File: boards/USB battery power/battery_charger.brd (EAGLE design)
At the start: 160 x 100 mm, 6 parts, among them IC1 MAX1555, U1 MAX8934EETI+, U2 LTC3127EMSEPBF

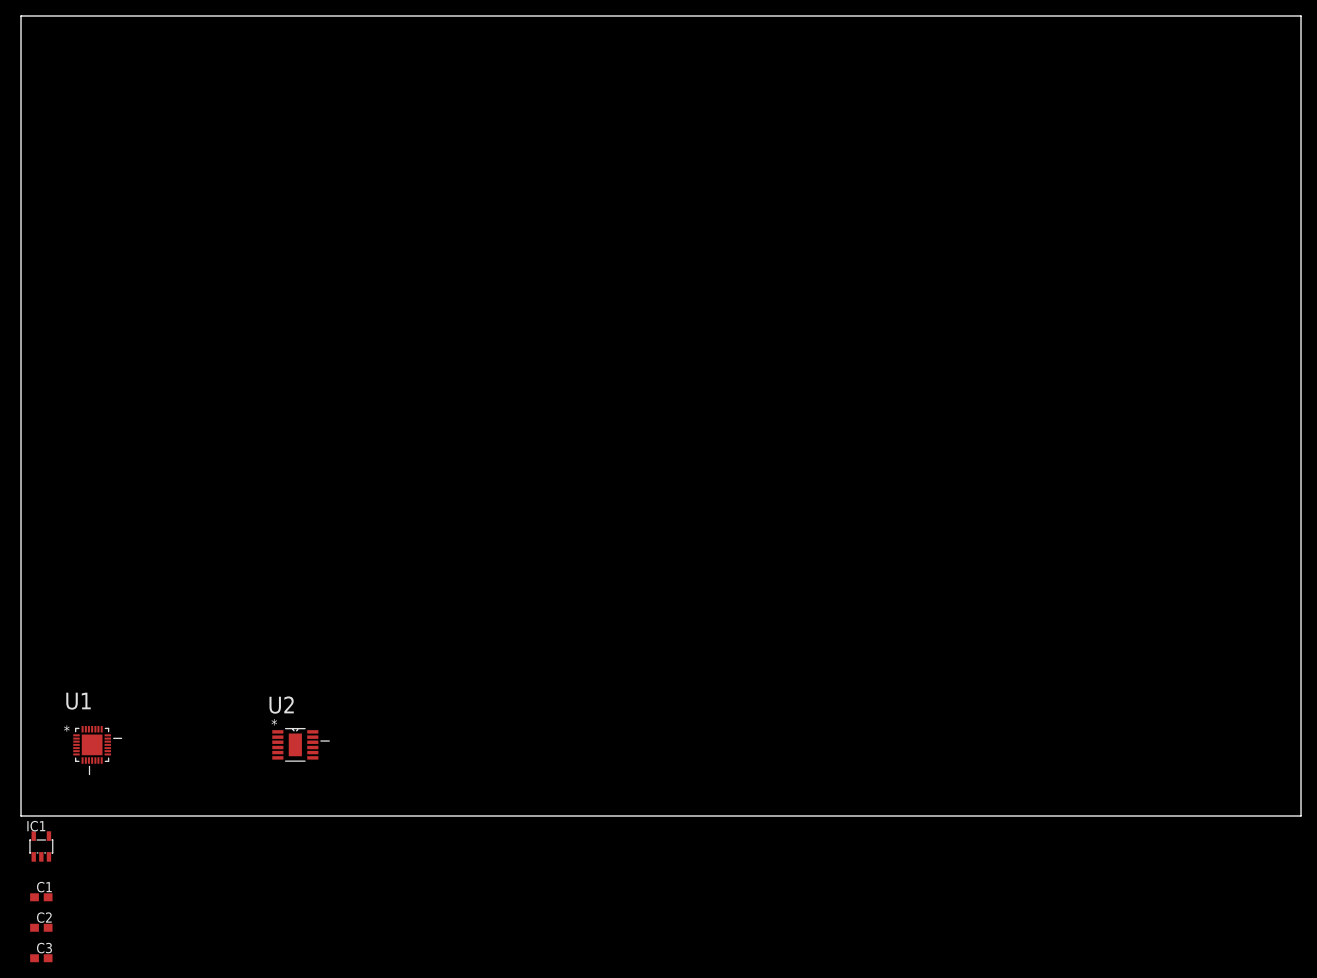
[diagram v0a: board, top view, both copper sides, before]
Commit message: Battery Charger test board
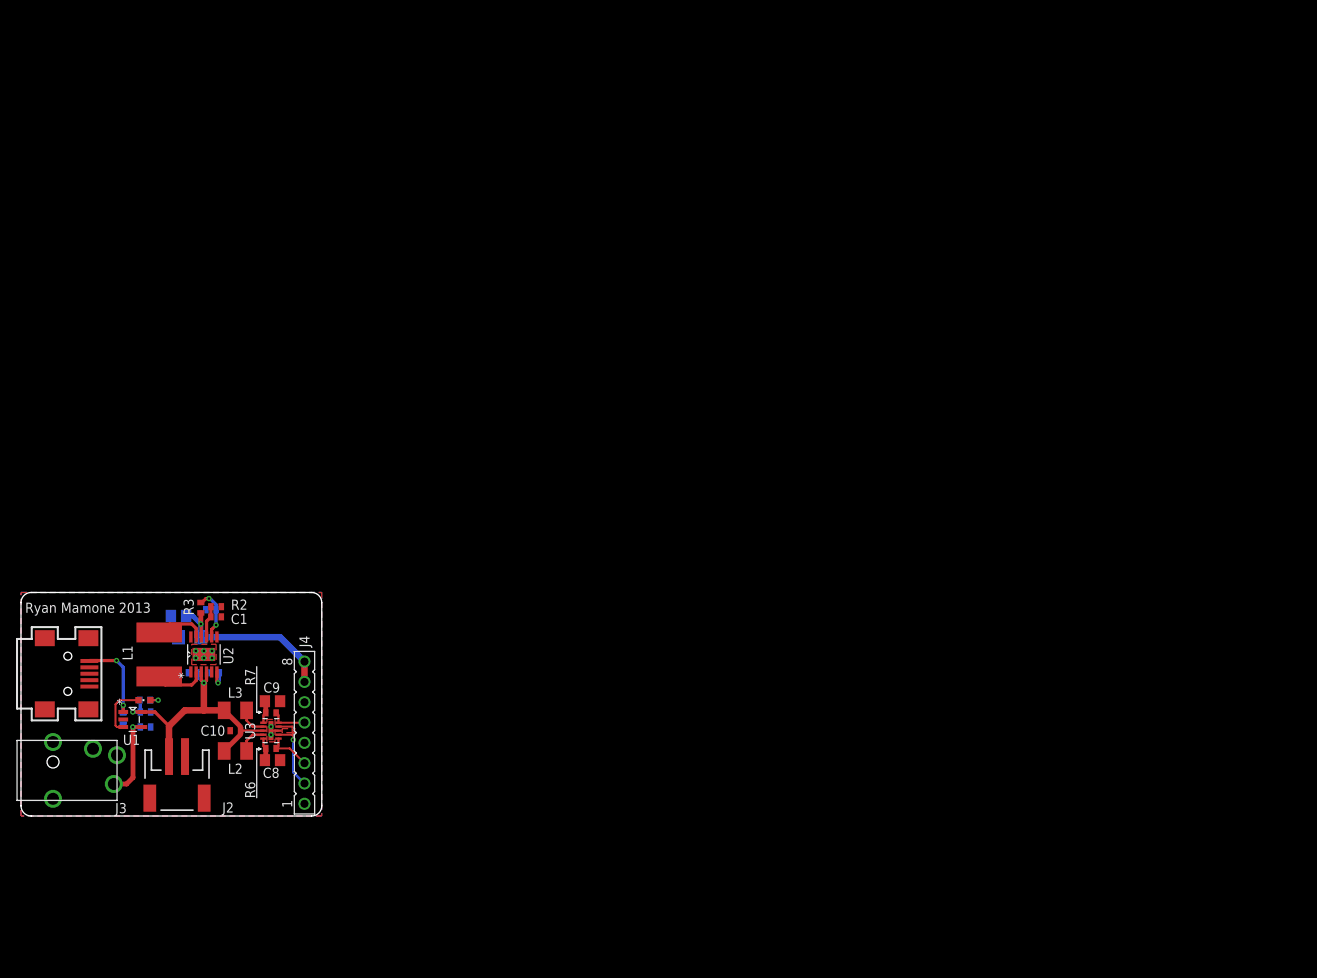
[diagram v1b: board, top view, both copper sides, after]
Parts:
- removed IC1: MAX1555, Maxim:SOT23-5L
- added C10, C5, C6, C7: 1uF, rcl:C0402
- added C4: 22uF, rcl:C0805
- added C8, C9: 1uF, rcl:C0805
- added J1: SAMTEC_MUSB, Custom:MUSB-05-X-B-SM-A
- added J2: JST_2MM_SMT, Custom:JST_2MM_SMT
- added J3: 5VDC, Custom:PJ-045
- added J4: IO, Custom:8-PIN_SIP_.100IN
- added L1: 4.7uH, Custom:NR6028
- added L2, L3: 15uH, rcl:L3225M
- added LED1: CHG, led:CHIPLED_0603
- added R1: 32.4k, rcl:R0402
- added R2: 499k, rcl:R0402
- added R3: 320k, rcl:R0402
- added R4: 182k, rcl:R0402
- added R5: 50, rcl:R0402
- added R6, R7: 10, rcl:R0402
- added U3: LT3497EDDBTRMPBF, LTC:DFN300X200X80-11N
- C1: value (none) -> 100pF; device rcl:C0603 -> rcl:C0402
- C2: value (none) -> 10uF; device rcl:C0603 -> rcl:C0402
- C3: value (none) -> 100uF; device rcl:C0603 -> rcl:C1206
- U1: value MAX8934EETI+ -> MAX1551EZK+T; device Maxim:QFN40P400X400X80-29N -> Maxim:SOT95P275X110-5N
- moved C3 44.2 mm to (21.1, 22.4), flipped to the bottom
- moved C1 41.3 mm to (24.4, 24.9)
- moved C2 37.1 mm to (21.6, 17.9), flipped to the bottom
- moved U2 16.1 mm to (22.9, 20.2), turned to 90 degrees
- moved U1 5.99 mm to (14.0, 12.1)
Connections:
- removed net +5V: C2.1, IC1.4
- removed net BATT: U1.21
- removed net BATT_2: U1.20
- removed net DC: U1.3
- removed net DC_2: U1.2
- removed net VIN: U2.3
- new net +3V3: C3.1, C4.1, J4.7, J4.8, R3.2, U2.10
- new net N$1: R1.2, U2.6
- new net N$10: J4.5, R7.1, U3.5
- new net N$11: C9.1, R7.2, U3.6
- new net N$12: L2.2, U3.9
- new net N$13: L3.2, U3.7
- new net N$14: J4.2, U3.2, U3.4
- new net N$2: R3.1, R4.2, U2.8
- new net N$3: L1.2, U2.2
- new net N$4: L1.1, U2.11
- new net N$5: LED1.C, U1.3
- new net N$6: C8.1, R6.2, U3.10
- new net N$7: C1.1, R2.2, U2.9
- new net N$8: LED1.A, R5.1
- new net N$9: J4.3, R6.1, U3.1
- new net V+: C5.1, J3.1, U1.4
- net +VBAT: now also C10.1, C2.1, C7.1, J2.2, L2.1, L3.1, R5.2, U1.5, U2.3, U2.4, U3.8; no longer C3.1, IC1.5
- net +VUSB: now also C6.1, J1.1, U1.1; no longer C1.1, IC1.1
- net GND: now also C10.2, C4.2, C5.2, C6.2, C7.2, C8.2, C9.2, J1.5, J2.1, J3.2, J3.3, J4.1, J4.4, J4.6, R1.1, R2.1, R4.1, U1.2, U2.1, U2.12, U2.13, U2.5, U2.7, U3.11, U3.3; no longer IC1.2
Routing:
- net +VBAT: track 0.00 -> 36.8 mm, vias 0 -> 2
- net +3V3: track 0.00 -> 23.7 mm, vias 0 -> 1
- net +VUSB: track 0.00 -> 12.1 mm, vias 0 -> 2
- net N$14: track 0.00 -> 11.5 mm, vias 0 -> 1
- net V+: track 0.00 -> 11.2 mm, vias 0 -> 1
- net N$2: track 0.00 -> 6.87 mm, vias 0 -> 2
- net N$5: track 0.00 -> 6.79 mm
- net N$3: track 0.00 -> 6.49 mm
- net N$4: track 0.00 -> 6.30 mm
- net N$9: track 0.00 -> 5.66 mm
- net N$10: track 0.00 -> 4.66 mm
- net N$7: track 0.00 -> 4.01 mm
- net N$13: track 0.00 -> 3.70 mm
- net N$12: track 0.00 -> 3.70 mm
- net N$11: track 0.00 -> 2.85 mm
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- added copper zone on layer 1, net GND
- added copper zone on layer 16, net GND
- added copper zone on layer 1, net N$18
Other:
- board size 160 x 100 mm -> 37.6 x 27.9 mm
- board text added: "Ryan Mamone 2013"
